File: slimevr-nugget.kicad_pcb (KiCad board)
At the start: 4 copper layers, 24 x 17.5 mm, 54 parts, among them U1 nRF52840-QFXX, U2 BQ24075RGT, U3 XC6220B331MR, U4 ICM-45686, U5 1532H, U6 QMC6309, Y1 32MHz

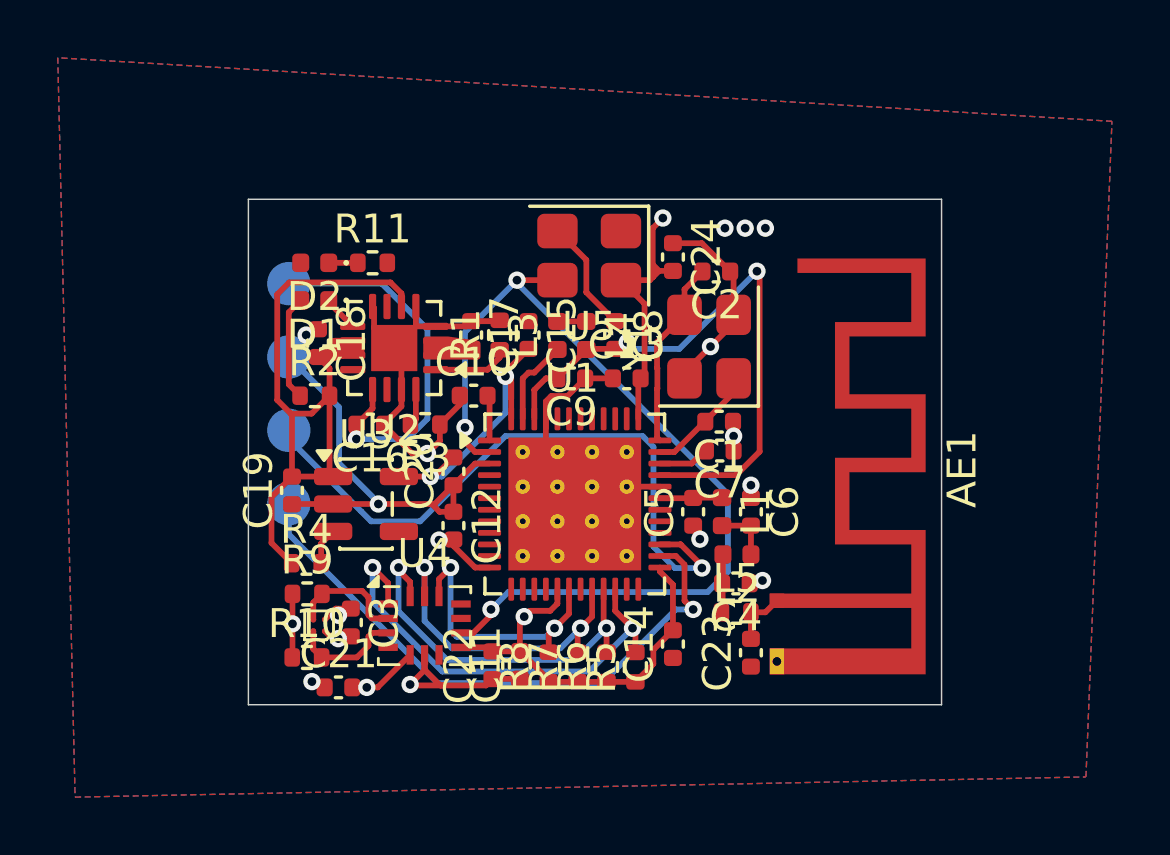
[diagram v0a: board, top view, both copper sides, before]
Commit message: Revision 2
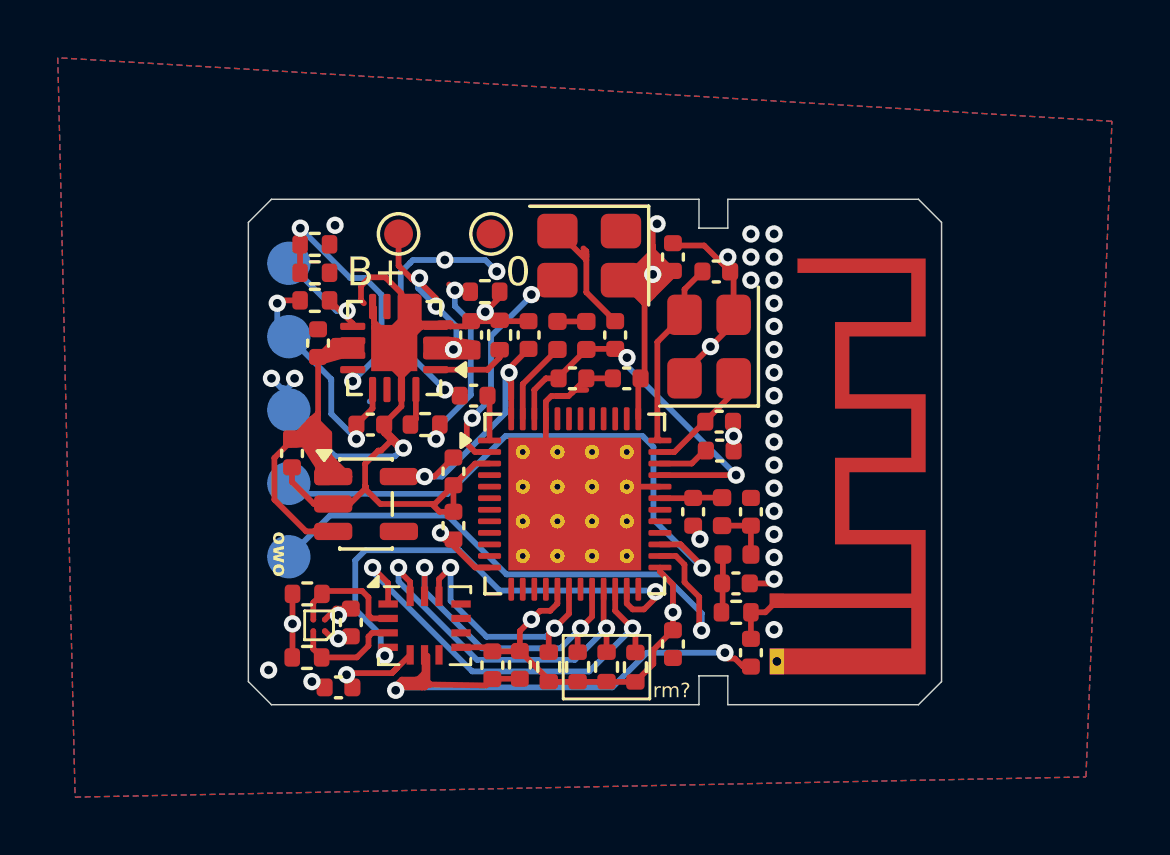
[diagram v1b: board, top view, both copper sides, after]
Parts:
- removed D1: ORANGE, LED_SMD:LED_0402_1005Metric
- removed D2: LED, LED_SMD:LED_0402_1005Metric
- removed U2: BQ24075RGT, Package_DFN_QFN:VQFN-16-1EP_3x3mm_P0.5mm_EP1.6x1.6mm
- added R12: 10k, Resistor_SMD:R_0402_1005Metric, F.Cu at (95.3, 140.1)
- added TP5: GND, TestPoint:TestPoint_Pad_D1.0mm, F.Cu at (101.4, 139.7)
- added TP6: BAT+, TestPoint:TestPoint_Pad_D1.0mm, F.Cu at (98.2, 139.7)
- added TP7: CHRG, TestPoint:TestPoint_Pad_D1.5mm, B.Cu at (94.4, 140.7)
- added U7: BQ24073RGT, Package_DFN_QFN:VQFN-16-1EP_3x3mm_P0.5mm_EP1.6x1.6mm, F.Cu at (98.0, 143.7)
- C24: value 1.0uF -> 100nF
- R4: value 10M -> 10k
- U4: value ICM-45686 -> LSM6DSV
- moved R4 11.2 mm to (101.2, 141.7), turned to 180 degrees
- moved R2 3.30 mm to (95.3, 142.0), turned to 180 degrees
- moved R11 2.03 mm to (95.3, 141.0), turned to 180 degrees
- moved TP1 1.84 mm to (94.4, 143.3)
- moved TP3 1.84 mm to (94.4, 148.3)
- moved TP4 1.84 mm to (94.4, 150.9)
- moved TP2 1.84 mm to (94.4, 145.8)
- moved C19 1.28 mm to (94.5, 147.3)
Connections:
- R11 pad 1: Net-(D2-K) -> GND
- R11 pad 2: GND -> Net-(U7-ILIM)
- R2 pad 1: Net-(D1-A) -> CHG
- R2 pad 2: VDDH -> VBUS
- R3 pad 1: GND -> Net-(R3-Pad1)
- R4 pad 1: VDDH -> GND
- R4 pad 2: PWRPIN -> Net-(R3-Pad1)
- U1 pad 13: PWRPIN -> unconnected-(U1-P0.13-Pad13)
- U1 pad 23: unconnected-(U1-P0.24-Pad23) -> INT1
- U3 pad 3: PWRPIN -> VDDH
- U4 pad 7: unconnected-(U4-GND-Pad7) -> GND
- U4 pad 9: CLK -> unconnected-(U4-INT2-Pad9)
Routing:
- net GND: track 58.0 -> 108.0 mm, vias 14 -> 37
- net CLK: track 32.2 -> 7.34 mm, vias 3 -> 2
- net VDD: track 42.2 -> 59.2 mm, vias 8 -> 10
- net INT1: track 0.00 -> 17.0 mm, vias 0 -> 2
- net Net-(U7-ILIM): track 0.00 -> 8.56 mm, vias 0 -> 2
- net Net-(U1-DEC4): track 20.8 -> 13.3 mm
- net Net-(R3-Pad1): track 0.00 -> 6.71 mm, vias 0 -> 2
- net BAT+: track 0.00 -> 6.63 mm, vias 0 -> 3
- net VDDH: track 24.0 -> 18.2 mm
- net VBUS: track 13.4 -> 9.33 mm, vias 1 -> 2
- net CHG: track 0.00 -> 4.03 mm, vias 0 -> 1
- net Net-(D1-A): track 3.63 -> 0.00 mm
- net SWC: track 22.8 -> 20.5 mm
- net PWRPIN: track 1.27 -> 0.00 mm
- net Net-(D1-K): track 1.24 -> 0.00 mm
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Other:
- outline, holes or cut-outs redrawn
- board text added: "0"
- board text added: "B+"
- board text added: "SWD SWC GND +5V CHG"
- board text added: "info's nugget"
- board text added: "owo"
- board text added: "rev.2"
- board text added: "rm?"
- board text removed: "SWD SWC GND +5V"
